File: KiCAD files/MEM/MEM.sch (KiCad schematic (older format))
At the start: 31 parts, among them J1 card addr, J2 Power Bus, J3 Signal Bus, J4 RAM bank, J5 ROM block, U1 74LS139, U2 74LS04, U3 74LS74, U4 74LS85, U5 SN74LS07N, U6 628128, U7 W27C512

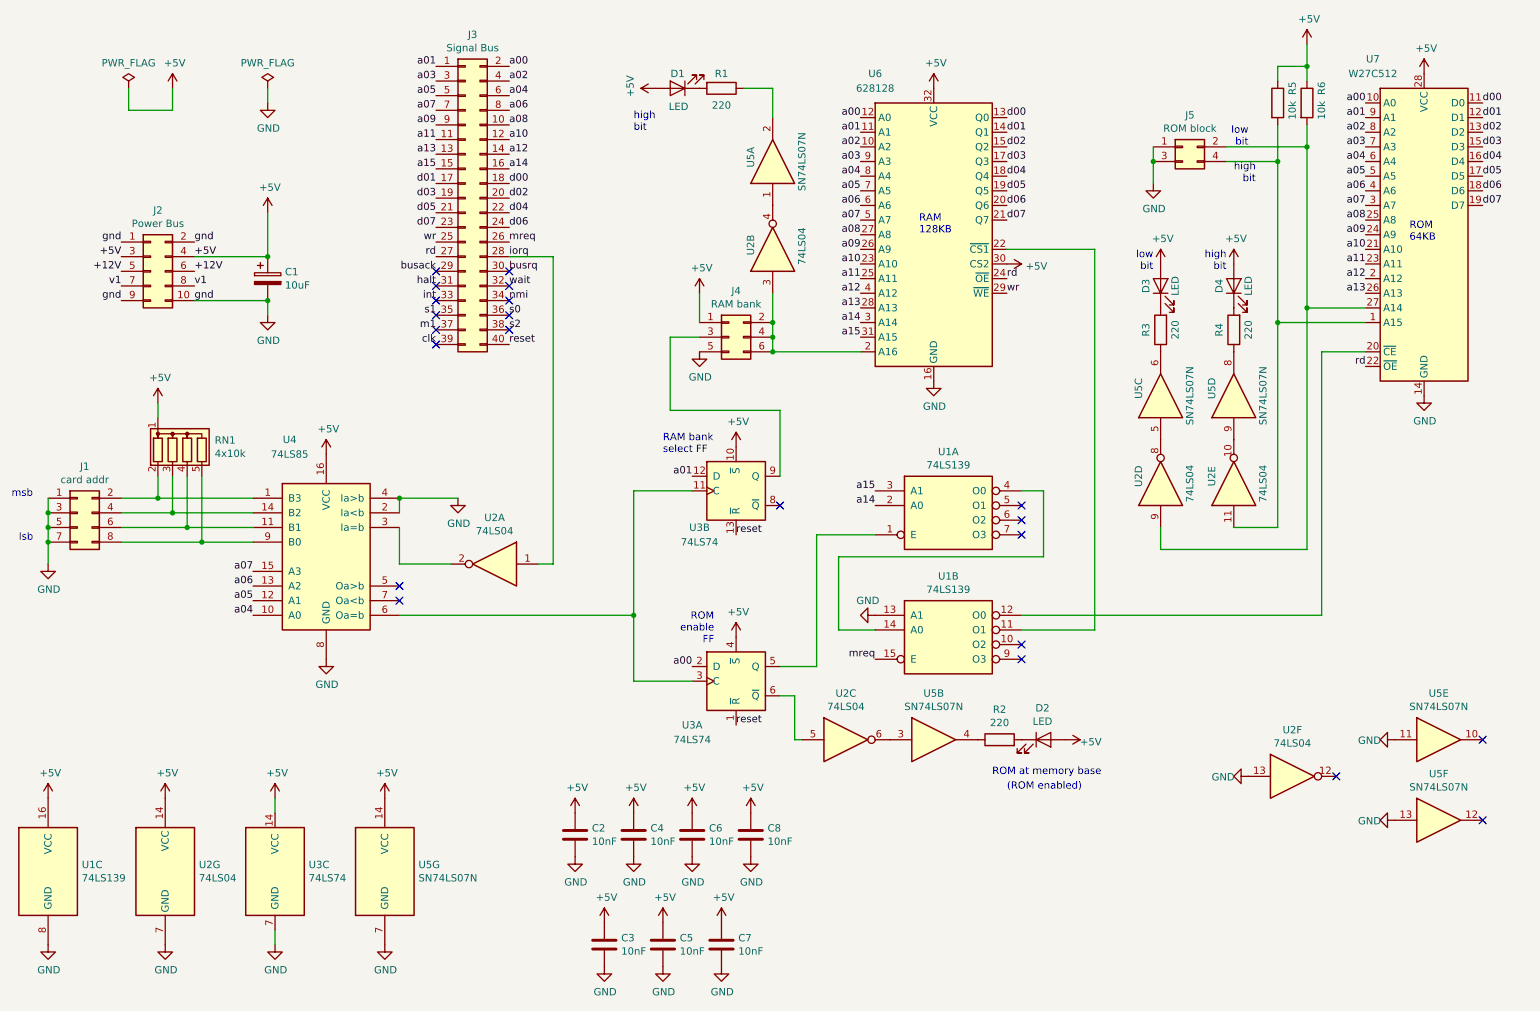
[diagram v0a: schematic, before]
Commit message: home
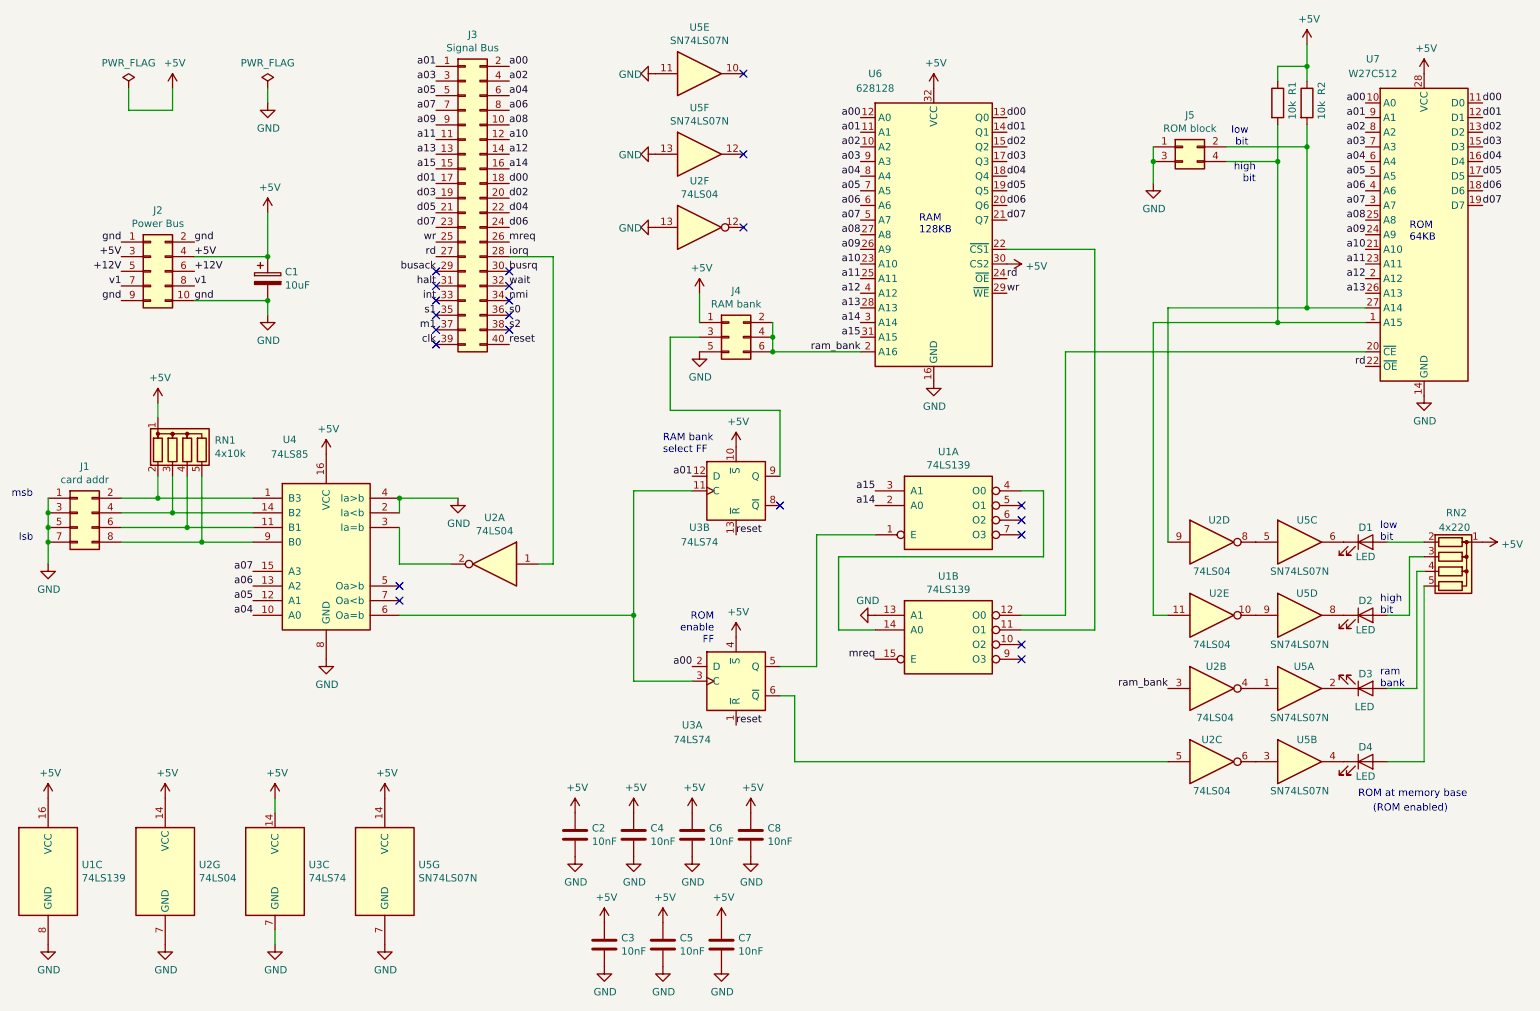
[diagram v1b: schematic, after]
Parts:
- removed R1, R2, R3, R4: 220, symbol Device:R
- added RN2: 4x220, Resistor_THT:R_Array_SIP5, symbol Device:R_Network04
- C1: footprint (none) -> Capacitor_THT:CP_Radial_D5.0mm_P2.50mm
- C2, C3, C4, C5, C6, C7, C8: footprint (none) -> Capacitor_THT:C_Disc_D3.8mm_W2.6mm_P2.50mm
- D1: renamed from D3; footprint (none) -> LED_THT:LED_D3.0mm
- D2: renamed from D4; footprint (none) -> LED_THT:LED_D3.0mm
- D3: renamed from D1; footprint (none) -> LED_THT:LED_D3.0mm
- D4: renamed from D2; footprint (none) -> LED_THT:LED_D3.0mm
- J1: footprint (none) -> Connector_PinHeader_2.54mm:PinHeader_2x04_P2.54mm_Vertical
- J2: footprint (none) -> Connector_PinHeader_2.54mm:PinHeader_2x05_P2.54mm_Vertical
- J3: footprint (none) -> Connector_PinHeader_2.54mm:PinHeader_2x20_P2.54mm_Vertical
- J4: footprint (none) -> Connector_PinSocket_2.54mm:PinSocket_2x03_P2.54mm_Vertical
- J5: footprint (none) -> Connector_PinHeader_2.54mm:PinHeader_2x02_P2.54mm_Vertical
- R1: renamed from R5; footprint (none) -> Resistor_THT:R_Axial_DIN0207_L6.3mm_D2.5mm_P10.16mm_Horizontal
- R2: renamed from R6; footprint (none) -> Resistor_THT:R_Axial_DIN0207_L6.3mm_D2.5mm_P10.16mm_Horizontal
- U1, U4: footprint (none) -> Package_DIP:DIP-16_W7.62mm_Socket_LongPads
- U2, U3, U5: footprint (none) -> Package_DIP:DIP-14_W7.62mm_Socket_LongPads
- U6: footprint (none) -> Package_DIP:DIP-32_W15.24mm_Socket_LongPads
- U7: footprint Package_DIP:DIP-28_W15.24mm -> Socket:DIP_Socket-28_W11.9_W12.7_W15.24_W17.78_W18.5_3M_228-1277-00-0602J
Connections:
- net +5V: now also RN2.1 (common); no longer D1.2 (A), D2.2 (A), D3.2 (A), D4.2 (A)
- net ram_bank: now reaches J4.2 (Pin_2), J4.4 (Pin_4), J4.6 (Pin_6), U2.3, U6.2 (A16)
- net at U5.4: now also D4.1 (K)
- net at D2.1 (K): now also U5.8
- net at D1.1 (K): now also U5.6
- net at D3.1 (K): now also U5.2
- new net: D4.2 (A), RN2.5 (R4)
- new net: D2.2 (A), RN2.3 (R2)
- new net: D1.2 (A), RN2.2 (R1)
- new net: D3.2 (A), RN2.4 (R3)
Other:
- note added: "ram\nbank"
- moved on the sheet: D1, D2, D3, D4, U2B, U2C, U2D, U2E, U2F, U5A, U5B, U5C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

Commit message: home
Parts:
- J4: footprint Connector_PinSocket_2.54mm:PinSocket_2x03_P2.54mm_Vertical -> Connector_PinHeader_2.54mm:PinHeader_2x03_P2.54mm_Vertical
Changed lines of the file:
@@
 F 0 "J4" H 5700 3167 50  0000 C CNN
 F 1 "RAM bank" H 5700 3076 50  0000 C CNN
-F 2 "Connector_PinSocket_2.54mm:PinSocket_2x03_P2.54mm_Vertical" H 5650 2850 50  0001 C CNN
+F 2 "Connector_PinHeader_2.54mm:PinHeader_2x03_P2.54mm_Vertical" H 5650 2850 50  0001 C CNN
 F 3 "~" H 5650 2850 50  0001 C CNN
 	1    5650 2850
